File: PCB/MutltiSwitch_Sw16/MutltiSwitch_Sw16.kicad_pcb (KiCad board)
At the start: 2 copper layers, 43 parts, among them IC1 ATMEGA328-P, P1 OUTPUT_9-16, P10 FTDI, P11 ICSP, P12 5v/6v, P13 DIODE2, P14 DIODE1, P15 SERVO, P16 GND_EXT, P17 ALIM_EXT2, P2 OUTPUT_9-16_ALIM, P3 SELECT_ALIM2, P4 OUTPUT_1-8, P5 OUTPUT_1-8_ALIM, P6 SELECT_ALIM1, P7 ALIM_EXT1, P8 XANY_INPUT, P9 OUTPUT_1-8_GND, U1 ULN2803, U2 ULN2803, X1 16Mhz

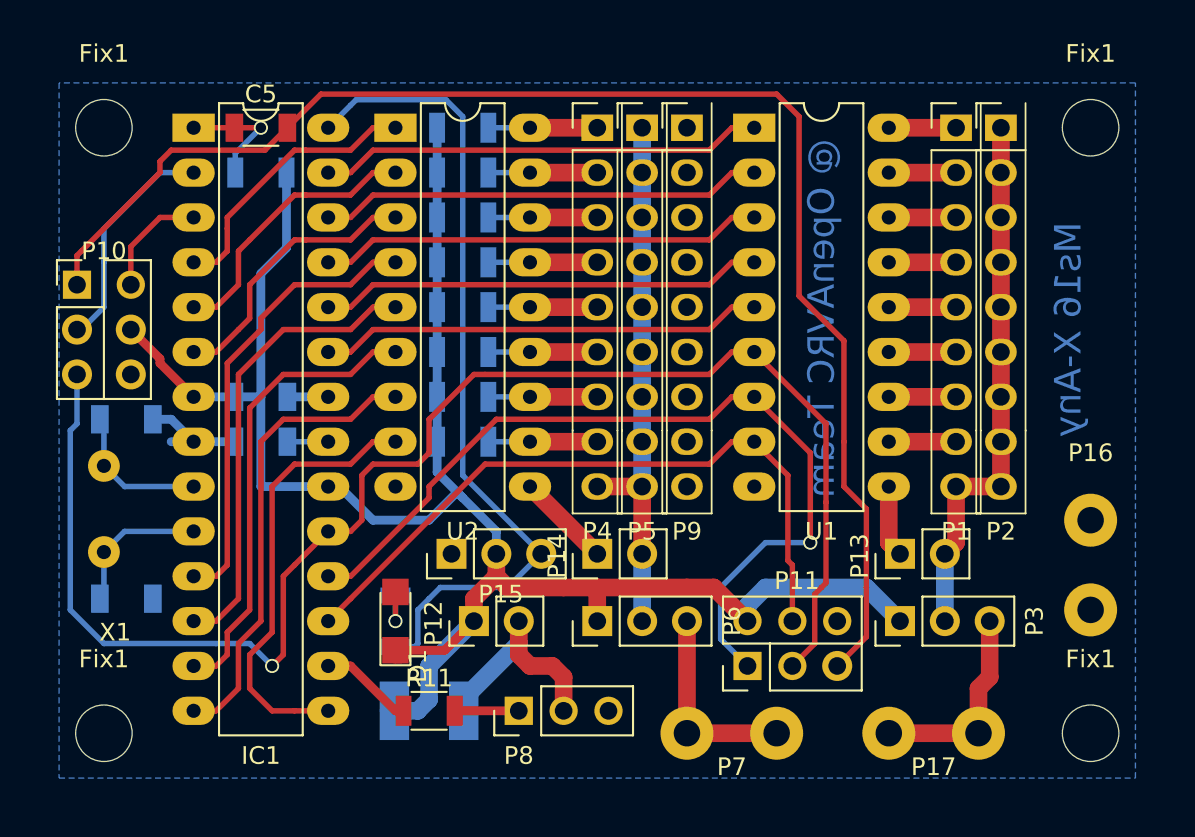
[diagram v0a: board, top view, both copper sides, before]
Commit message: Update_PCB_Multiswitch_16
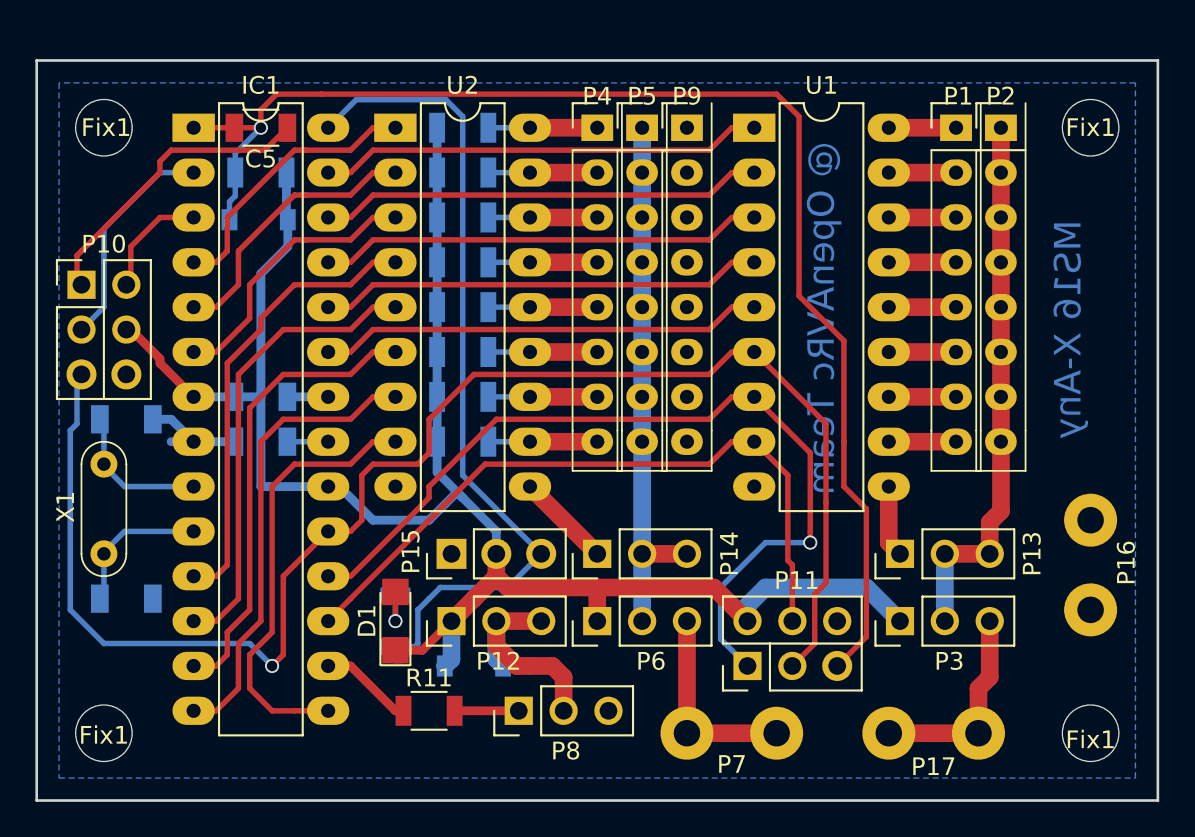
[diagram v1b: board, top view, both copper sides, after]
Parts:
- added D3: LL4148, mylib:D_SOD-123, B.Cu at (145.9, 78.9)
- C1, C2, C3, C4, C5: footprint C_1206 -> mylib:C_1206
- D1: footprint LED_1206 -> mylib:LED_1206
- D2: value 1N4001 -> LL4148; footprint D_DO-204AC -> mylib:D_SOD-123
- IC1: footprint DIP-28_W7.62mm_LongPads -> mylib:DIP-28_W7.62mm_LongPads
- P1, P2, P4, P5, P9: footprint Pin_Header_Straight_1x09_Pitch2.54mm -> mylib:Pin_Header_Straight_1x08_Pitch2.54mm
- P10, P11: footprint Pin_Header_Straight_2x03_Pitch2.54mm -> mylib:Pin_Header_Straight_2x03_Pitch2.54mm
- P12: value 5v/6v -> +V = VRx / +V < VRx; footprint Pin_Header_Straight_1x02_Pitch2.54mm -> mylib:Pin_Header_Straight_1x03_Pitch2.54mm
- P13, P14: footprint Pin_Header_Straight_1x02_Pitch2.54mm -> mylib:Pin_Header_Straight_1x03_Pitch2.54mm
- P16: footprint Faston_V-5_08 -> mylib:Faston_V-5_08
- P17: value ALIM_EXT2 -> VExt2; footprint Faston_V-5_08 -> mylib:Faston_V-5_08
- P3: value SELECT_ALIM2 -> SEL_ALIM2; footprint Pin_Header_Straight_1x03_Pitch2.54mm -> mylib:Pin_Header_Straight_1x03_Pitch2.54mm
- P6: value SELECT_ALIM1 -> SEL_ALIM1; footprint Pin_Header_Straight_1x03_Pitch2.54mm -> mylib:Pin_Header_Straight_1x03_Pitch2.54mm
- P7: value ALIM_EXT1 -> VExt1; footprint Faston_V-5_08 -> mylib:Faston_V-5_08
- P8: footprint Pin_Header_Straight_1x03_Pitch2.54mm -> mylib:Pin_Header_Straight_1x03_Pitch2.54mm
- R1, R10, R11, R3, R4, R5, R6, R7, R8, R9: footprint R_1206 -> mylib:R_1206
- R2: value 10K -> 330; footprint R_1206 -> mylib:R_1206
- U1, U2: footprint DIP-18_W7.62mm_LongPads -> mylib:DIP-18_W7.62mm_LongPads
- X1: footprint HC-39 -> mylib:HC-39
- moved D2 3.59 mm to (158.1, 104.1)
- moved P12 1.27 mm to (156.8, 101.6)
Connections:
- P11 pad 5: Net-(C5-Pad2) -> Net-(C5-Pad1)
- P13 pad 2: Net-(P1-Pad9) -> Net-(P13-Pad2)
- P2 pad 1: Net-(P1-Pad9) -> Net-(P13-Pad2)
- P2 pad 2: Net-(P1-Pad9) -> Net-(P13-Pad2)
- P2 pad 3: Net-(P1-Pad9) -> Net-(P13-Pad2)
- P2 pad 4: Net-(P1-Pad9) -> Net-(P13-Pad2)
- P2 pad 5: Net-(P1-Pad9) -> Net-(P13-Pad2)
- P2 pad 6: Net-(P1-Pad9) -> Net-(P13-Pad2)
- P2 pad 7: Net-(P1-Pad9) -> Net-(P13-Pad2)
- P2 pad 8: Net-(P1-Pad9) -> Net-(P13-Pad2)
- P3 pad 2: Net-(P1-Pad9) -> Net-(P13-Pad2)
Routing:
- net Net-(C5-Pad1): track 6.95 -> 75.5 mm
- net Net-(C5-Pad2): track 80.6 -> 16.9 mm
- net Net-(P1-Pad9): track 30.7 -> 0.00 mm
- net Net-(P13-Pad2): track 0.00 -> 30.7 mm
- net +5V: track 113.0 -> 106.0 mm
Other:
- board outline added: 63.5 x 41.9 mm
- board text added: "8x10K"
- board text added: "@ OpenAVRc Team"
- board text added: "MS16 X-Any"
- board text removed: "8x1K"
- board text removed: "@ OpenAVRC Team"
- board text removed: "Ms16 X-Any"
